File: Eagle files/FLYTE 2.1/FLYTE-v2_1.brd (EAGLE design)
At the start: 116 x 55 mm, 88 parts, among them Q1 IRF540NPBF, Q2 IRF540NPBF, U3 ADS1115IDGSR, U6 W25Q32JVSSIQ

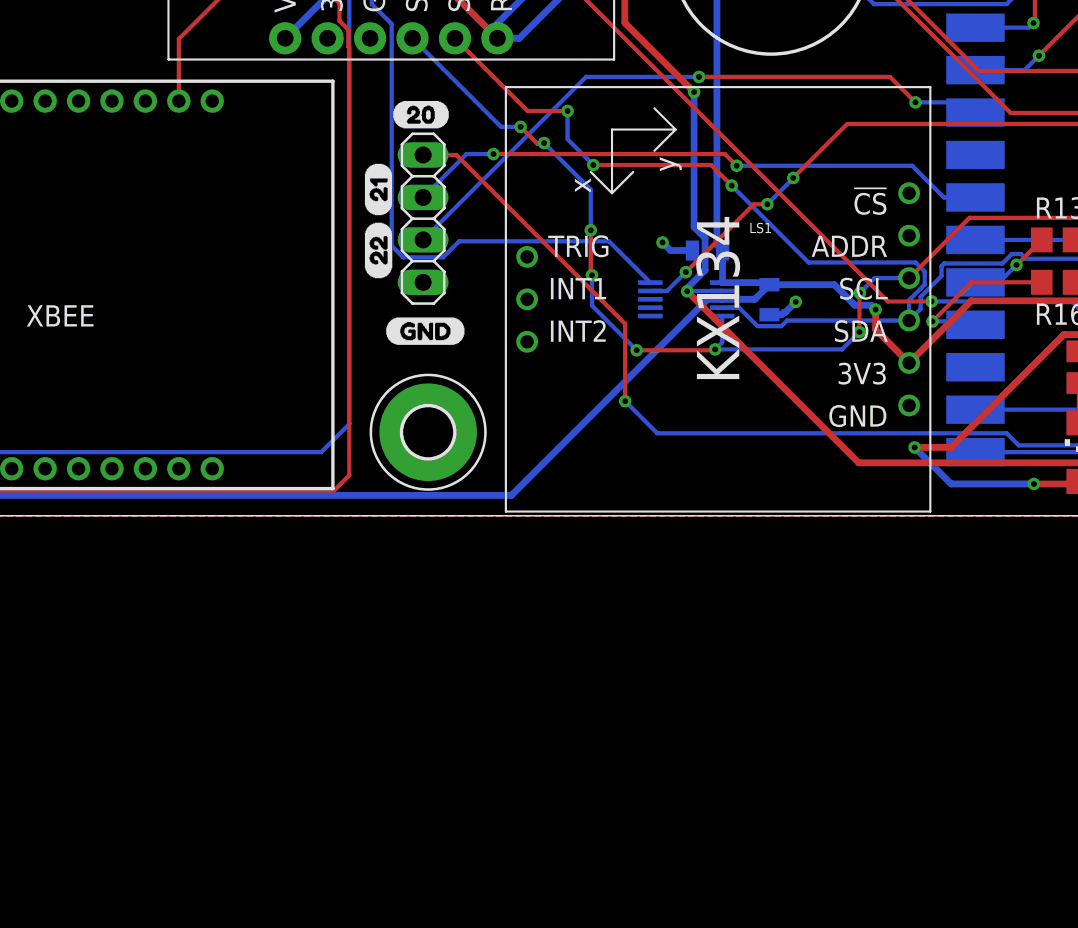
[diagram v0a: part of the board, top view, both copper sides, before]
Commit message: reefing
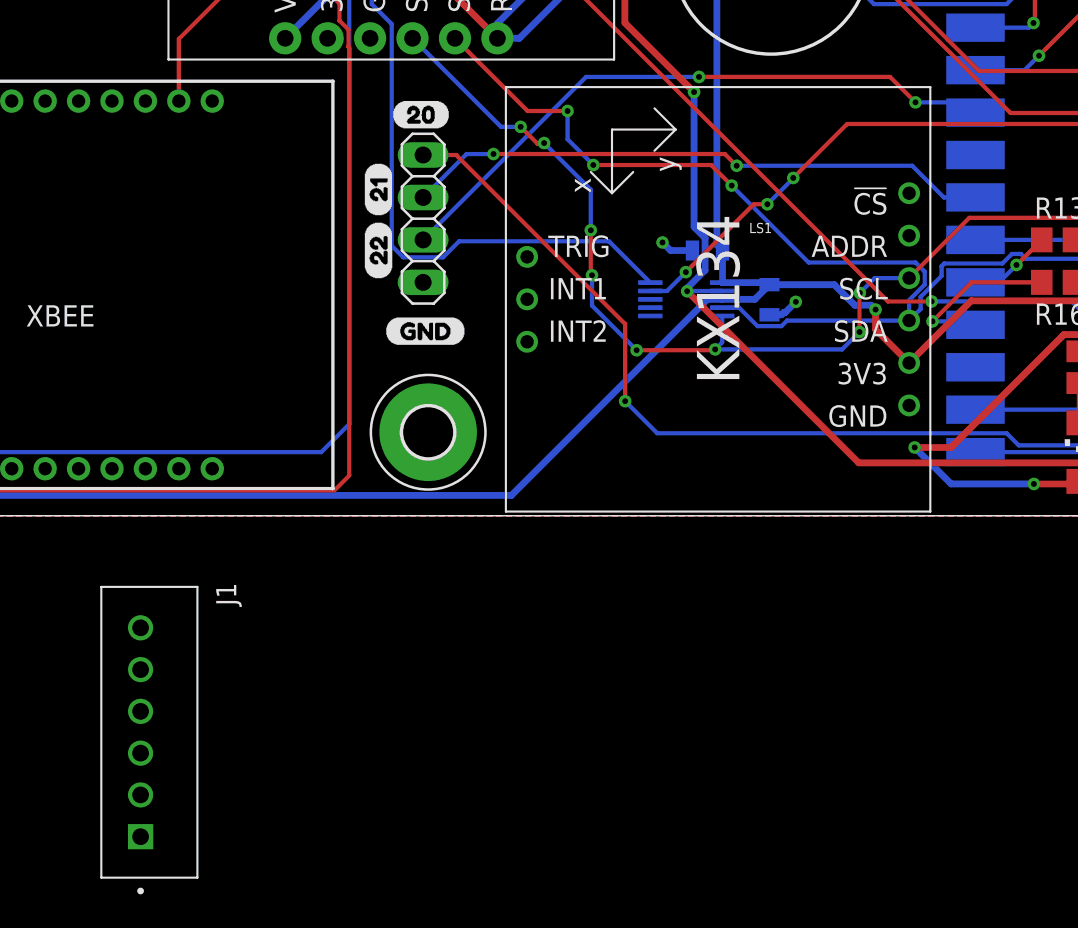
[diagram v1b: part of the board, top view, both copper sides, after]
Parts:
- added J1: B6B-XH-A(LF)(SN), B6B-XH-A_LF__SN_:JST_B6B-XH-A(LF)(SN)
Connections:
- removed net 22: JP3.3, U1.P$29
- new net CS_TEMP: J1.2, JP3.3, U1.P$29
- new net TEMP_VOUT: J1.5
- net 3V3: now also J1.6
- net GND: now also J1.4
- net MISO1: now also J1.3
- net SCK1: now also J1.1
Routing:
- net 22: track 38.0 -> 0.00 mm, vias 2 -> 0
- net CS_TEMP: track 0.00 -> 37.1 mm, vias 0 -> 2
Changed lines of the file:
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@@
 <element name="U$26" library="vbus_label" package="VBUS0" value="" x="116.205" y="51.816" smashed="yes" rot="R90"/>
 <element name="U$27" library="flyte_label" package="FLYTE_V2#10" value="" x="124.3965" y="45.9105" smashed="yes"/>
+<element name="J1" library="B6B-XH-A_LF__SN_" package="JST_B6B-XH-A(LF)(SN)" override_package3d_urn="urn:adsk.eagle:package:44254739/2" override_package_urn="urn:adsk.eagle:footprint:44254740/1" value="B6B-XH-A(LF)(SN)" x="67.437" y="4.953" smashed="yes" rot="R270">
+<attribute name="CHECK_PRICES" value="https://www.snapeda.com/parts/B6B-XH-A(LF)(SN)/JST+Sales+America+Inc./view-part/?ref=eda" x="67.437" y="4.953" size="1.778" layer="27" rot="R270" display="off"/>
+<attribute name="DESCRIPTION" value=" Connector Header Through Hole 6 position 0.098 (2.50mm) " x="67.437" y="4.953" size="1.778" layer="27" rot="R270" display="off"/>
+<attribute name="MF" value="JST Sales" x="67.437" y="4.953" size="1.778" layer="27" rot="R270" display="off"/>
+<attribute name="MP" value="B6B-XH-A(LF)(SN)" x="67.437" y="4.953" size="1.778" layer="27" rot="R270" display="off"/>
+<attribute name="NAME" x="71.437" y="13.903" size="1.2" layer="25" ratio="18" rot="R270"/>
+<attribute name="PACKAGE" value="None" x="67.437" y="4.953" size="1.778" layer="27" rot="R270" display="off"/>
+<attribute name="SNAPEDA_LINK" value="https://www.snapeda.com/parts/B6B-XH-A(LF)(SN)/JST+Sales+America+Inc./view-part/?ref=snap" x="67.437" y="4.953" size="1.778" layer="27" rot="R270" display="off"/>
+<attribute name="VALUE" x="62.437" y="13.903" size="1.2" layer="27" ratio="18" rot="R270"/>
+</element>
 </elements>
 <signals>
@@
 <wire x1="105.39703125" y1="30.0736" x2="105.4862" y2="30.0736" width="0.4064" layer="16"/>
 <wire x1="105.4862" y1="30.0736" x2="106.1212" y2="30.7086" width="0.4064" layer="16"/>
+<contactref element="J1" pad="4"/>
+<wire x1="151.0515" y1="57.277" x2="157.863" y2="67.907" width="0" layer="19" extent="1-1"/>
+<wire x1="150.561" y1="49.657" x2="151.0515" y2="57.277" width="0" layer="19" extent="16-16"/>
+<wire x1="155.194" y1="45.659" x2="150.561" y2="49.657" width="0" layer="19" extent="16-16"/>
+<wire x1="160.418" y1="40.707" x2="155.194" y2="45.659" width="0" layer="19" extent="16-16"/>
+<wire x1="154.178" y1="35.477" x2="160.418" y2="40.707" width="0" layer="19" extent="16-16"/>
+<wire x1="148.209" y1="30.11" x2="154.178" y2="35.477" width="0" layer="19" extent="16-16"/>
+<wire x1="152.284" y1="26.162" x2="148.209" y2="30.11" width="0" layer="19" extent="16-16"/>
+<wire x1="157.863" y1="22.907" x2="152.284" y2="26.162" width="0" layer="19" extent="16-16"/>
+<wire x1="141.843" y1="31.877" x2="148.209" y2="30.11" width="0" layer="19" extent="16-16"/>
+<wire x1="136.873" y1="26.797" x2="141.843" y2="31.877" width="0" layer="19" extent="16-16"/>
+<wire x1="140.843" y1="22.987" x2="136.873" y2="26.797" width="0" layer="19" extent="16-16"/>
+<wire x1="130.683" y1="27.747" x2="136.873" y2="26.797" width="0" layer="19" extent="1-16"/>
+<wire x1="126.873" y1="27.747" x2="130.683" y2="27.747" width="0" layer="19" extent="1-1"/>
+<wire x1="123.063" y1="27.747" x2="126.873" y2="27.747" width="0" layer="19" extent="1-1"/>
+<wire x1="116.873" y1="26.797" x2="123.063" y2="27.747" width="0" layer="19" extent="1-16"/>
+<wire x1="112.903" y1="24.511" x2="116.873" y2="26.797" width="0" layer="19" extent="16-16"/>
+<wire x1="112.903" y1="34.671" x2="116.873" y2="26.797" width="0" layer="19" extent="16-16"/>
+<wire x1="116.873" y1="39.497" x2="112.903" y2="34.671" width="0" layer="19" extent="16-16"/>
+<wire x1="106.1212" y1="30.7086" x2="112.903" y2="34.671" width="0" layer="19" extent="1-1"/>
+<wire x1="99.938" y1="33.782" x2="104.5464" y2="29.9356" width="0" layer="19" extent="16-16"/>
+<wire x1="97.418" y1="30.861" x2="98.1456" y2="34.2646" width="0" layer="19" extent="16-16"/>
+<wire x1="97.418" y1="29.861" x2="97.418" y2="30.861" width="0" layer="19" extent="16-16"/>
+<wire x1="136.873" y1="39.497" x2="141.843" y2="31.877" width="0" layer="19" extent="16-16"/>
+<wire x1="141.843" y1="42.037" x2="136.873" y2="39.497" width="0" layer="19" extent="16-16"/>
+<wire x1="136.873" y1="52.197" x2="141.843" y2="42.037" width="0" layer="19" extent="16-16"/>
+<wire x1="132.6134" y1="58.166" x2="136.873" y2="52.197" width="0" layer="19" extent="16-16"/>
+<wire x1="136.873" y1="64.897" x2="133.314" y2="61.617" width="0" layer="19" extent="1-16"/>
+<wire x1="133.314" y1="70.717" x2="136.873" y2="64.897" width="0" layer="19" extent="1-16"/>
+<wire x1="125.3236" y1="57.8866" x2="132.6134" y2="58.166" width="0" layer="19" extent="1-1"/>
+<wire x1="124.932" y1="70.717" x2="133.314" y2="70.717" width="0" layer="19" extent="1-1"/>
+<wire x1="116.873" y1="64.897" x2="124.932" y2="61.617" width="0" layer="19" extent="1-16"/>
+<wire x1="108.723" y1="61.087" x2="116.873" y2="64.897" width="0" layer="19" extent="16-16"/>
+<wire x1="103.113" y1="61.087" x2="108.723" y2="61.087" width="0" layer="19" extent="16-16"/>
+<wire x1="102.358" y1="58.717" x2="103.113" y2="61.087" width="0" layer="19" extent="16-16"/>
+<wire x1="97.293" y1="61.087" x2="102.358" y2="58.717" width="0" layer="19" extent="16-16"/>
+<wire x1="92.833" y1="58.717" x2="97.293" y2="61.087" width="0" layer="19" extent="16-16"/>
+<wire x1="91.683" y1="61.087" x2="92.833" y2="58.717" width="0" layer="19" extent="16-16"/>
+<wire x1="85.725" y1="64.262" x2="91.683" y2="61.087" width="0" layer="19" extent="16-16"/>
+<wire x1="83.185" y1="64.262" x2="85.725" y2="64.262" width="0" layer="19" extent="1-1"/>
+<wire x1="80.645" y1="64.262" x2="83.185" y2="64.262" width="0" layer="19" extent="1-1"/>
+<wire x1="78.934" y1="69.388" x2="80.645" y2="64.262" width="0" layer="19" extent="1-1"/>
+<wire x1="87.904" y1="69.388" x2="85.725" y2="64.262" width="0" layer="19" extent="1-1"/>
+<wire x1="107.529" y1="70.104" x2="108.723" y2="61.087" width="0" layer="19" extent="16-16"/>
+<wire x1="116.873" y1="52.197" x2="125.3236" y2="57.8866" width="0" layer="19" extent="16-16"/>
+<wire x1="83.82" y1="31.877" x2="97.418" y2="30.861" width="0" layer="19" extent="16-16"/>
+<wire x1="84.121" y1="22.907" x2="83.82" y2="31.877" width="0" layer="19" extent="1-1"/>
+<wire x1="71.2006" y1="20.7246" x2="84.121" y2="22.907" width="0" layer="19" extent="1-1"/>
+<wire x1="80.645" y1="46.482" x2="83.82" y2="31.877" width="0" layer="19" extent="1-1"/>
+<wire x1="66.912" y1="6.203" x2="71.2006" y2="20.7246" width="0" layer="19" extent="1-1"/>
+<wire x1="60.386" y1="59.944" x2="80.645" y2="64.262" width="0" layer="19" extent="16-16"/>
+<wire x1="58.6255" y1="52.324" x2="60.386" y2="59.944" width="0" layer="19" extent="16-16"/>
+<wire x1="53.0352" y1="47.2338" x2="58.6255" y2="52.324" width="0" layer="19" extent="16-16"/>
+<wire x1="51.863" y1="67.907" x2="60.386" y2="59.944" width="0" layer="19" extent="16-16"/>
 </signal>
 <signal name="VCC">
@@
 <wire x1="109.855" y1="63.5" x2="109.728" y2="63.627" width="0.4064" layer="1"/>
 <wire x1="107.453" y1="63.627" x2="109.728" y2="63.627" width="0.4064" layer="16"/>
+<contactref element="J1" pad="6"/>
+<wire x1="53.2006" y1="20.7246" x2="66.912" y2="11.203" width="0" layer="19" extent="1-1"/>
 </signal>
 <signal name="BUZZER">
@@
 <wire x1="139.7856" y1="31.39303125" x2="140.147" y2="31.03163125" width="0.254" layer="16"/>
 <wire x1="140.147" y1="31.03163125" x2="140.147" y2="29.718" width="0.254" layer="16"/>
+<contactref element="J1" pad="3"/>
+<wire x1="66.912" y1="3.703" x2="136.873" y2="31.877" width="0" layer="19" extent="16-16"/>
 </signal>
 <signal name="SCK1">
@@
 <wire x1="152.2174" y1="28.9676" x2="152.2174" y2="29.12396875" width="0.254" layer="16"/>
 <wire x1="152.2174" y1="29.12396875" x2="143.21596875" y2="38.1254" width="0.254" layer="16"/>
+<contactref element="J1" pad="1"/>
+<wire x1="66.912" y1="-1.297" x2="136.873" y2="36.957" width="0" layer="19" extent="16-16"/>
 </signal>
 <signal name="MOSI1">
@@
 <wire x1="122.743" y1="31.877" x2="125.123" y2="31.877" width="0.254" layer="1"/>
 </signal>
-<signal name="22">
-<contactref element="U1" pad="P$29"/>
-<contactref element="JP3" pad="3"/>
-<wire x1="83.82" y1="34.417" x2="93.5736" y2="44.1706" width="0.254" layer="16"/>
-<wire x1="93.5736" y1="44.1706" x2="100.33" y2="44.1706" width="0.254" layer="16"/>
-<via x="100.33" y="44.1706" extent="1-16" drill="0.35"/>
-<wire x1="100.33" y1="44.1706" x2="111.76" y2="44.1706" width="0.254" layer="1"/>
-<wire x1="111.76" y1="44.1706" x2="113.284" y2="42.6466" width="0.254" layer="1"/>
-<via x="113.284" y="42.6466" extent="1-16" drill="0.35"/>
-<wire x1="113.284" y1="42.6466" x2="116.2634" y2="42.6466" width="0.254" layer="16"/>
-<wire x1="116.2634" y1="42.6466" x2="116.873" y2="42.037" width="0.254" layer="16"/>
-</signal>
 <signal name="21">
 <contactref element="U1" pad="P$27"/>
@@
 <contactref element="U$2" pad="INT2"/>
 </signal>
+<signal name="TEMP_VOUT">
+<contactref element="J1" pad="5"/>
+</signal>
+<signal name="CS_TEMP">
+<contactref element="U1" pad="P$29"/>
+<contactref element="JP3" pad="3"/>
+<wire x1="83.82" y1="34.417" x2="93.5736" y2="44.1706" width="0.254" layer="16"/>
+<wire x1="93.5736" y1="44.1706" x2="100.33" y2="44.1706" width="0.254" layer="16"/>
+<via x="100.33" y="44.1706" extent="1-16" drill="0.35"/>
+<wire x1="100.33" y1="44.1706" x2="111.76" y2="44.1706" width="0.254" layer="1"/>
+<wire x1="111.76" y1="44.1706" x2="113.284" y2="42.6466" width="0.254" layer="1"/>
+<via x="113.284" y="42.6466" extent="1-16" drill="0.35"/>
+<wire x1="113.284" y1="42.6466" x2="116.2634" y2="42.6466" width="0.254" layer="16"/>
+<contactref element="J1" pad="2"/>
+<wire x1="116.2634" y1="42.6466" x2="116.873" y2="42.037" width="0" layer="19" extent="16-16"/>
+<wire x1="66.912" y1="1.203" x2="83.82" y2="34.417" width="0" layer="19" extent="1-1"/>
+</signal>
 </signals>

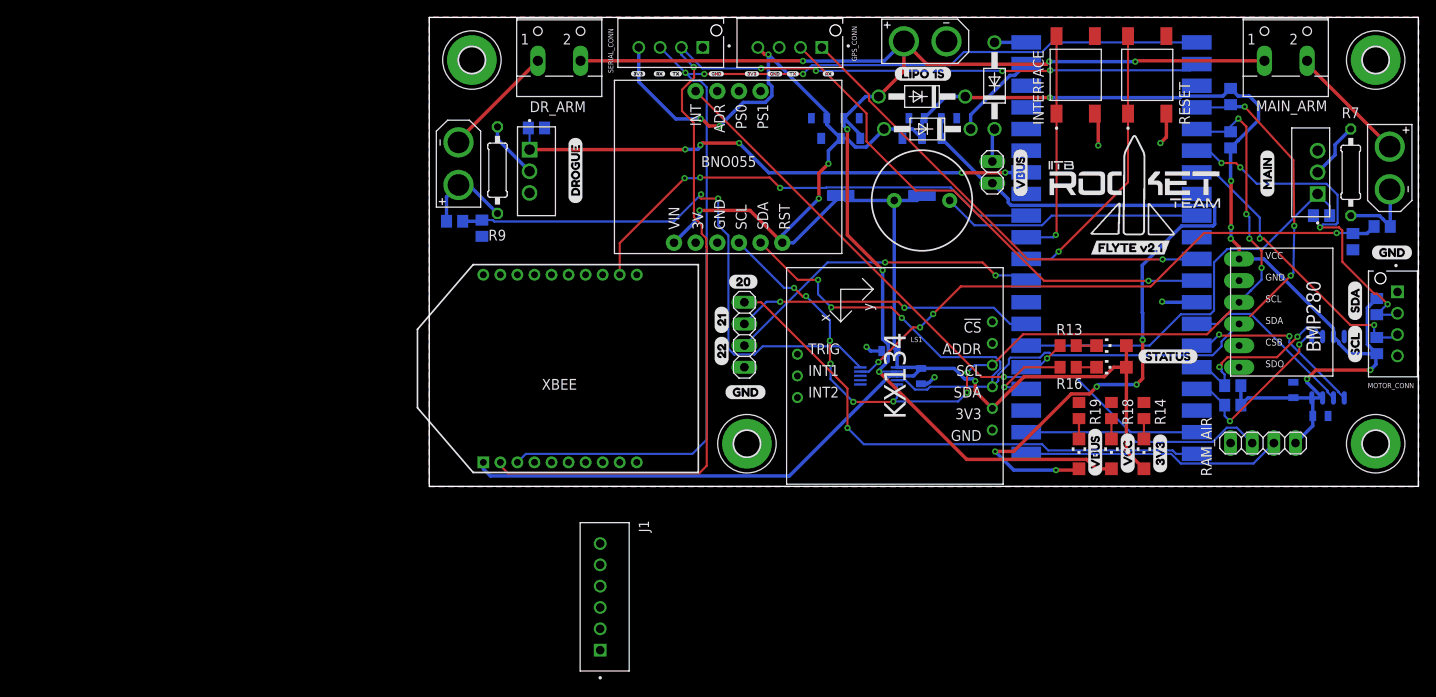
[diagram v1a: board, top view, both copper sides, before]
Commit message: oof
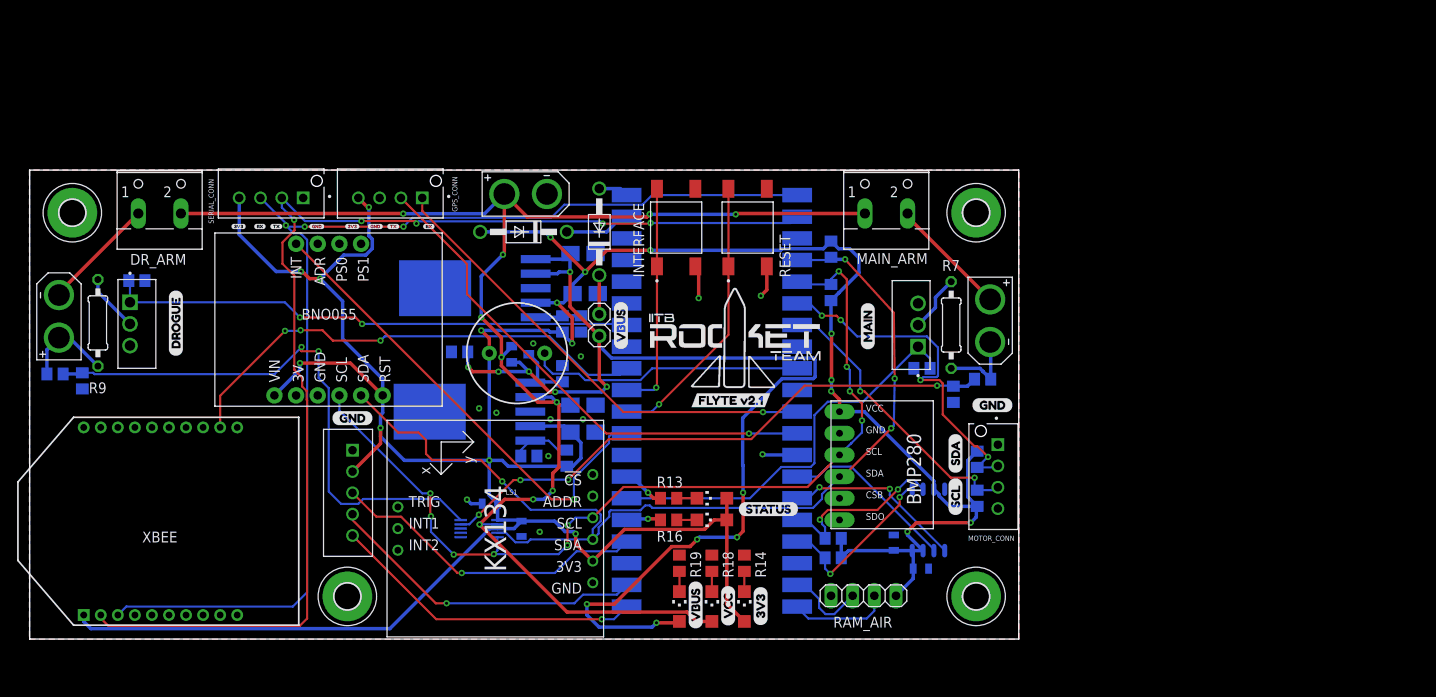
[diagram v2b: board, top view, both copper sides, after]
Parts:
- removed C1, C2, C3, C4: 22uF, SparkFun-Capacitors:0805
- removed D2: 1N4004, diode:DO41-10
- removed JP3: (no value), pinhead:1X04
- removed LIPO_REG, USB_REG: AMS1117-3.3, AMS1117-3.3:SOT229P700X180-4N
- removed U$14: (no value), lipo_1s_label:LIPO_1S0
- removed U$6: (no value), 20_label:200
- removed U$7: (no value), 21_label:210
- removed U$8: (no value), 22_label:220
- added C11, C6: 10uF, microbuilder:EIA3216-18/A-W
- added C12, C7: 10 uF, microbuilder:EIA3216-18/A-W
- added Q3: (no value), microbuilder:SOT23-WIDE
- added R10, R21: 165K ohm, rcl:R0805
- added R20, R8: 100K ohm, rcl:R0805
- added R22, R24: 4.7K ohm, rcl:R0805
- added U2, U4: MIC29302WU-TR, MIC29302WU:TO-263-5_MCH
- J1: value B6B-XH-A(LF)(SN) -> B5B-XH-A(LF)(SN); device B6B-XH-A_LF__SN_:JST_B6B-XH-A(LF)(SN) -> B5B-XH-A_LF__SN_:JST_B5B-XH-A(LF)(SN)
- moved LS1 50.8 mm to (57.1, 33.5)
- moved Q2 50.2 mm to (103.4, 36.8)
- moved R17 50.2 mm to (94.2, 11.8)
- moved U$15 50.2 mm to (110.5, 27.4)
- moved U$17 50.2 mm to (108.6, 19.4)
- moved C10 50.2 mm to (57.7, 12.9)
- moved R15 50.2 mm to (94.2, 9.53)
- moved U$16 50.2 mm to (108.6, 14.5)
- moved 3V3_LED 50.2 mm to (83.8, 3.81)
- moved C8 50.2 mm to (101.3, 11.3)
- moved DROGUE 50.2 mm to (3.43, 37.8)
- moved DR_ARM 50.2 mm to (15.2, 51.2)
- moved H1 50.2 mm to (5.00, 50.0)
- moved H3 50.2 mm to (111.0, 50.0)
- moved H4 50.2 mm to (111.0, 5.00)
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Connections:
- removed net 20: JP3.1, U1.P$20
- removed net 21: JP3.2, U1.P$27
- removed net TEMP_VOUT: J1.5
- new net MISO0: J1.5, U1.P$21
- new net N$10: R10.2, R8.1, U2.5
- new net N$5: R20.1, R21.2, U4.5
- new net SCK0: J1.3, U1.P$24
- new net VCC_EN: Q3.3, R22.2, U4.1
- net 3V3: now also C12.+, C7.+, J1.2, R10.1, R21.1, U2.4, U4.4; no longer C1.2, C3.2, D2.C, J1.6, LIPO_REG.2, LIPO_REG.4, USB_REG.2, USB_REG.4
- net AIR_DATA: now also U1.P$20; no longer U1.P$21
- net AIR_SCK: now also U1.P$19; no longer U1.P$22
- net BNO_INT: now also U1.P$29; no longer U1.P$19
- net CS_TEMP: now also J1.4, U1.P$22; no longer J1.2, JP3.3, U1.P$29
- net GND: now also C11.-, C12.-, C6.-, C7.-, J1.1, R20.2, R22.1, R24.1, R8.2, U2.3, U2.6, U4.3, U4.6; no longer C1.1, C2.1, C3.1, C4.1, J1.4, JP3.4, LIPO_REG.1, USB_REG.1
- net LED1: now also U1.P$27; no longer U1.P$25
- net LED2: now also U1.P$25; no longer U1.P$24
- net MISO1: no longer J1.3
- net SCK1: no longer J1.1
- net VBUS_REG: now also C6.+, Q3.1, R24.2, U2.1, U2.2; no longer C4.2, USB_REG.3
- net VCC: now also C11.+, Q3.2, U4.2; no longer C2.2, D2.A, LIPO_REG.3
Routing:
- net 20: track 63.1 -> 0.00 mm, vias 1 -> 0
- net VBUS_REG: track 95.4 -> 135.7 mm, vias 5 -> 11
- net SCK0: track 0.00 -> 37.6 mm, vias 0 -> 1
- net MISO0: track 0.00 -> 36.8 mm, vias 0 -> 1
- net 21: track 35.2 -> 0.00 mm, vias 2 -> 0
- net 3V3: track 354.8 -> 389.8 mm, vias 13 -> 18
- net BNO_INT: track 75.3 -> 56.3 mm
- net AIR_SCK: track 28.4 -> 9.42 mm
- net AIR_DATA: track 30.5 -> 11.8 mm
- net VCC: track 164.9 -> 175.0 mm, vias 6 -> 10
- net VCC_EN: track 0.00 -> 7.47 mm
- net N$5: track 0.00 -> 7.00 mm
- net LED2: track 10.2 -> 4.08 mm
- net N$10: track 0.00 -> 5.36 mm
- net N$1: track 10.6 -> 7.75 mm
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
